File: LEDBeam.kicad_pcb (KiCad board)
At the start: 2 copper layers, 67.3 x 71.1 mm, 12 parts, among them J1 Power, J2 Switch, J3 Power led, U1 WeMos_D1_mini, U2 LED_Dimmer_Platine, U3 LED_Dimmer_Platine, U4 LM7805_TO220, U5 LED_Dimmer_Platine, U6 LED_Dimmer_Platine

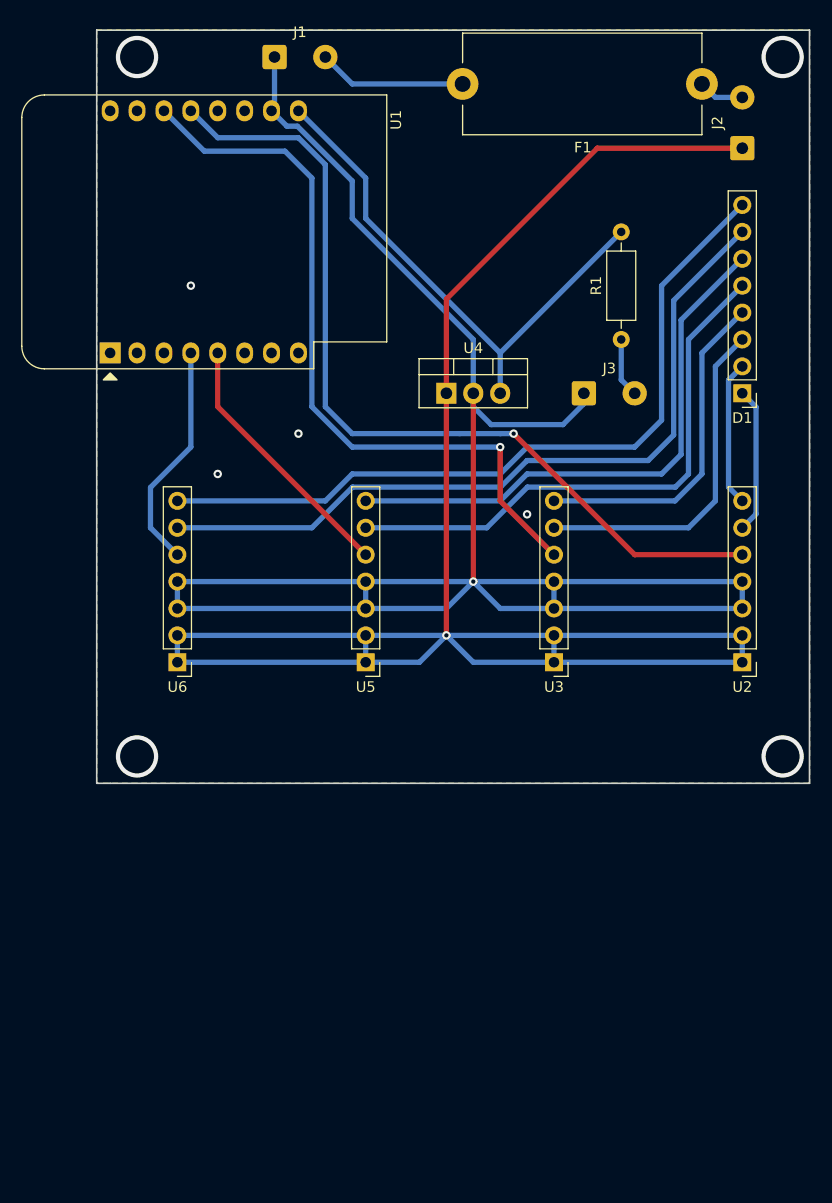
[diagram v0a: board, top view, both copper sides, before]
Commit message: New board design
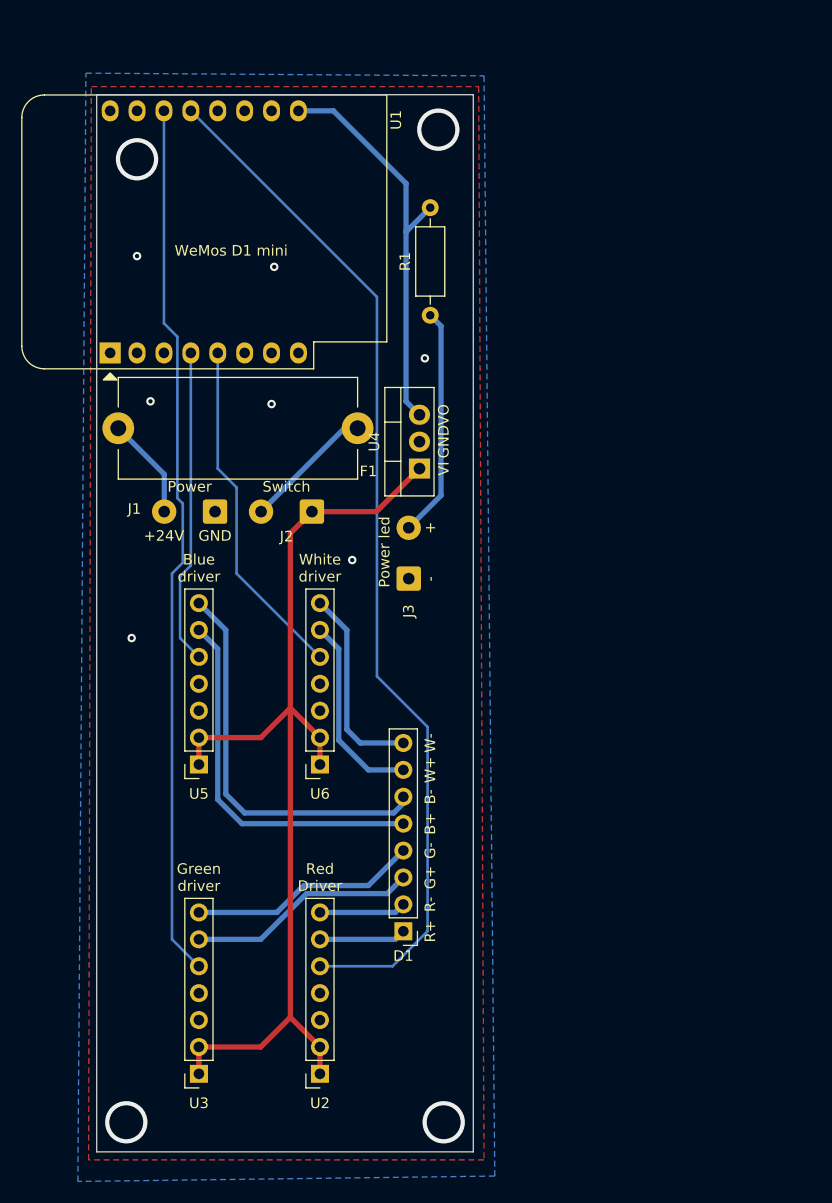
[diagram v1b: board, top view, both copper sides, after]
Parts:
- U2, U3, U5, U6: footprint Connector_PinHeader_2.54mm:PinHeader_1x07_P2.54mm_Vertical -> LEDBeam:LED_Driver_module
- moved D1 60.0 mm to (39.1, 129.5)
- moved U2 55.7 mm to (31.2, 143.0)
- moved J2 53.2 mm to (30.5, 89.9), turned to 180 degrees
- moved U3 51.3 mm to (19.8, 143.0)
- moved F1 46.0 mm to (34.8, 82.0)
- moved J1 43.3 mm to (21.3, 89.9), turned to 180 degrees
- moved J3 24.1 mm to (39.6, 96.2), turned to 90 degrees
- moved U5 18.5 mm to (19.8, 113.8)
- moved R1 18.2 mm to (41.7, 71.4)
- moved U6 16.6 mm to (31.2, 113.8)
- moved U4 7.55 mm to (40.6, 85.9), turned to 90 degrees
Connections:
- net 24V renamed +24V
- net 5V renamed +5V
- U1 pad 4: W_PWM -> B_PWM
- U1 pad 5: B_PWM -> W_PWM
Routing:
- net GND: track 191.3 -> 0.40 mm, vias 5 -> 7
- net +24V: track 184.5 -> 98.1 mm, vias 1 -> 0
- net W+: track 72.4 -> 18.4 mm
- net W-: track 72.4 -> 18.9 mm
- net B+: track 52.5 -> 35.2 mm
- net Net-(J3-Pad2): track 5.61 -> 21.7 mm
- net R_PWM: track 82.8 -> 98.3 mm, vias 1 -> 0
- net B-: track 52.5 -> 37.6 mm
- net G_PWM: track 69.8 -> 83.0 mm, vias 1 -> 0
- net +5V: track 50.7 -> 38.6 mm
- net W_PWM: track 21.7 -> 32.7 mm
- net G+: track 32.6 -> 21.7 mm
- net G-: track 31.8 -> 21.7 mm
- net Net-(F1-Pad1): track 4.34 -> 12.4 mm
- net R-: track 13.8 -> 8.19 mm
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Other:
- board size 67.3 x 71.1 mm -> 35.6 x 99.8 mm
- board text added: "+"
- board text added: "+24V"
- board text added: "-"
- board text added: "B+"
- board text added: "B-"
- board text added: "Blue driver"
- board text added: "G+"
- board text added: "G-"
- board text added: "GND"
- board text added: "Green driver"
- board text added: "R+"
- board text added: "R-"
- board text added: "Red Driver"
- board text added: "VI"
- board text added: "VO"
- board text added: "W+"
- board text added: "W-"
- board text added: "WeMos D1 mini"
- board text added: "White driver"
